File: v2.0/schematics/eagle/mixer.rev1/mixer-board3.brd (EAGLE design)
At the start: 100 x 80 mm, 64 parts, among them IC1 TL082P, IC2 TL082P, IC3 TL082P, IC4 TL082P, J1 RTN-2, J2 RTN-1, J3 SEND1, J4 SEND2

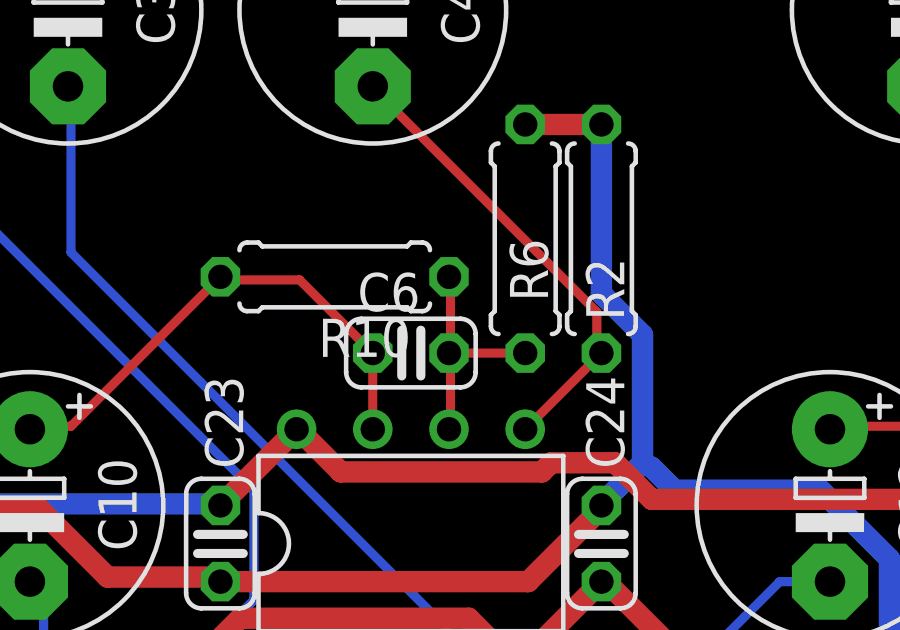
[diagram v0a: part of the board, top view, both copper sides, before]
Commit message: Board corrections
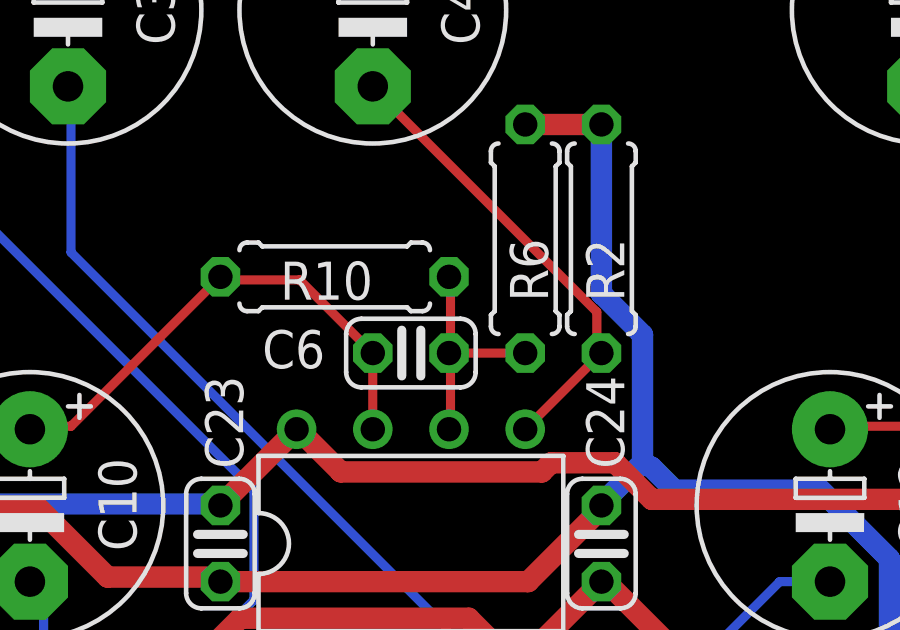
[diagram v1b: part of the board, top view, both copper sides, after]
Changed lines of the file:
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@@
 <grid distance="50" unitdist="mil" unit="mm" style="lines" multiple="1" display="yes" altdistance="0.635" altunitdist="mm" altunit="mm"/>
 <layers>
-<layer number="1" name="Top" color="4" fill="1" visible="yes" active="yes"/>
-<layer number="16" name="Bottom" color="1" fill="1" visible="yes" active="yes"/>
+<layer number="1" name="Top" color="4" fill="1" visible="no" active="yes"/>
+<layer number="16" name="Bottom" color="1" fill="1" visible="no" active="yes"/>
 <layer number="17" name="Pads" color="2" fill="1" visible="yes" active="yes"/>
 <layer number="18" name="Vias" color="2" fill="1" visible="yes" active="yes"/>
@@
 </element>
 <element name="C6" library="_common" package="C025-024X044" value="22pF" x="62.23" y="38.1" smashed="yes">
-<attribute name="NAME" x="60.452" y="39.497" size="1.27" layer="25" ratio="10"/>
+<attribute name="NAME" x="57.277" y="37.592" size="1.27" layer="25" ratio="10"/>
 <attribute name="VALUE" x="60.452" y="35.433" size="1.27" layer="27" ratio="10"/>
 </element>
@@
 </element>
 <element name="R10" library="_common" package="0207/7" value="30k" x="59.69" y="40.64" smashed="yes" rot="R180">
-<attribute name="NAME" x="62.23" y="39.243" size="1.27" layer="25" ratio="10" rot="R180"/>
+<attribute name="NAME" x="60.96" y="41.148" size="1.27" layer="25" ratio="10" rot="R180"/>
 <attribute name="VALUE" x="61.976" y="41.1988" size="1.27" layer="27" ratio="10" rot="R180"/>
 </element>
@@
 </element>
 <element name="R2" library="_common" package="0207/7" value="10K" x="68.58" y="41.91" smashed="yes" rot="R270">
-<attribute name="NAME" x="68.072" y="41.275" size="1.27" layer="25" ratio="10" rot="R270"/>
+<attribute name="NAME" x="68.072" y="41.91" size="1.27" layer="25" ratio="10" rot="R270"/>
 <attribute name="VALUE" x="68.0212" y="44.196" size="1.27" layer="27" ratio="10" rot="R270"/>
 </element>
